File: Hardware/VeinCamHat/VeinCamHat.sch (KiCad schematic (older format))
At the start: 23 parts, among them J1 Raspberry_Pi_2_3, Q1 BSD235N

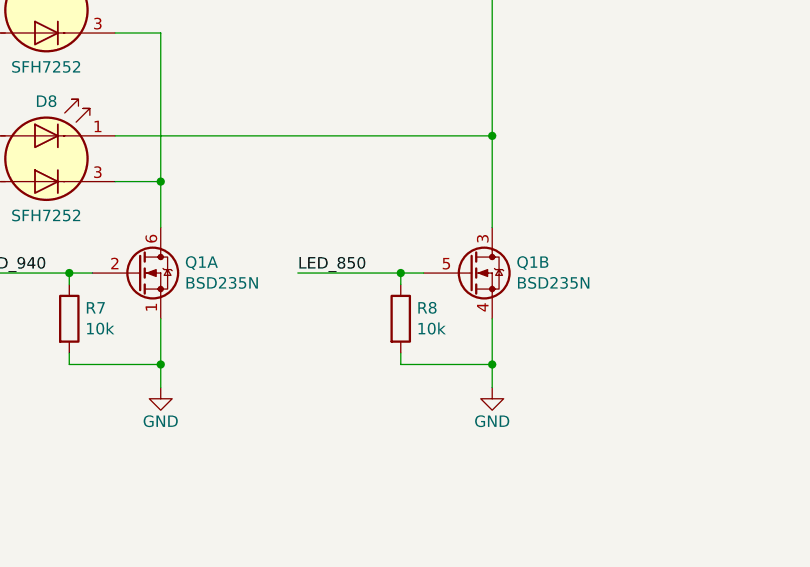
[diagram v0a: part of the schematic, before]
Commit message: More Hardware changes, both boards complete
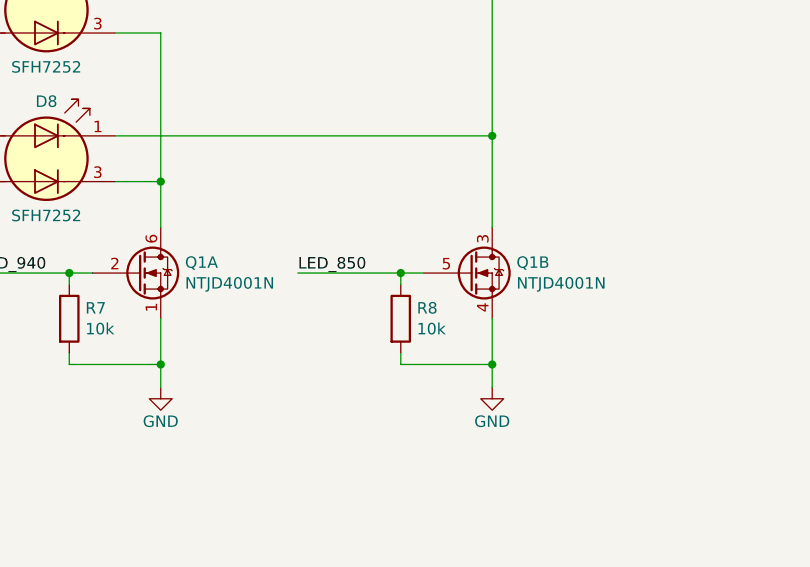
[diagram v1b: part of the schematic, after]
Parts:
- removed Q1: BSD235N, Package_TO_SOT_SMD:SOT-363_SC-70-6, symbol VeinCam_Symbols:BSD235N
- added Q1: NTJD4001N, Package_TO_SOT_SMD:SOT-363_SC-70-6, symbol VeinCam_Symbols:NTJD4001N
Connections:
- net GND: now also Q1.1 (S), Q1.4 (S)
- net LED_850: now also Q1.5 (G)
- net LED_940: now also Q1.2 (G)
- net at D7.3 (K1), D8.3 (K1): now also Q1.6 (D)
- net at D7.1 (K2), D8.1 (K2): now also Q1.3 (D)
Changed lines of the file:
@@
 	4600 2250 4850 2250
-$Comp
-L VeinCam_Symbols:BSD235N Q1
-U 1 1 5C89B330
-P 8900 2950
-F 0 "Q1" H 9106 2996 50  0000 L CNN
-F 1 "BSD235N" H 9106 2905 50  0000 L CNN
-F 2 "Package_TO_SOT_SMD:SOT-363_SC-70-6" H 9100 2950 50  0001 C CNN
-F 3 "~" H 9100 2950 50  0001 C CNN
-	1    8900 2950
-	1    0    0    -1
-$EndComp
-$Comp
-L VeinCam_Symbols:BSD235N Q1
-U 2 1 5C89B4BB
-P 10350 2950
-F 0 "Q1" H 10556 2996 50  0000 L CNN
-F 1 "BSD235N" H 10556 2905 50  0000 L CNN
-F 2 "Package_TO_SOT_SMD:SOT-363_SC-70-6" H 10550 2950 50  0001 C CNN
-F 3 "~" H 10550 2950 50  0001 C CNN
-	2    10350 2950
-	1    0    0    -1
-$EndComp
 $Comp
 L VeinCam_Symbols:SFH7252 D3
@@
 NoConn ~ 2650 1950
 NoConn ~ 2650 2050
+$Comp
+L VeinCam_Symbols:NTJD4001N Q1
+U 1 1 5C91E58D
+P 8900 2950
+F 0 "Q1" H 9106 2996 50  0000 L CNN
+F 1 "NTJD4001N" H 9106 2905 50  0000 L CNN
+F 2 "Package_TO_SOT_SMD:SOT-363_SC-70-6" H 9100 2950 50  0001 C CNN
+F 3 "~" H 9100 2950 50  0001 C CNN
+	1    8900 2950
+	1    0    0    -1
+$EndComp
+$Comp
+L VeinCam_Symbols:NTJD4001N Q1
+U 2 1 5C91E612
+P 10350 2950
+F 0 "Q1" H 10556 2996 50  0000 L CNN
+F 1 "NTJD4001N" H 10556 2905 50  0000 L CNN
+F 2 "Package_TO_SOT_SMD:SOT-363_SC-70-6" H 10550 2950 50  0001 C CNN
+F 3 "~" H 10550 2950 50  0001 C CNN
+	2    10350 2950
+	1    0    0    -1
+$EndComp
 $EndSCHEMATC
